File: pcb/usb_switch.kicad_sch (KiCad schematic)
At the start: 1 part, among them U2 FE1.1s

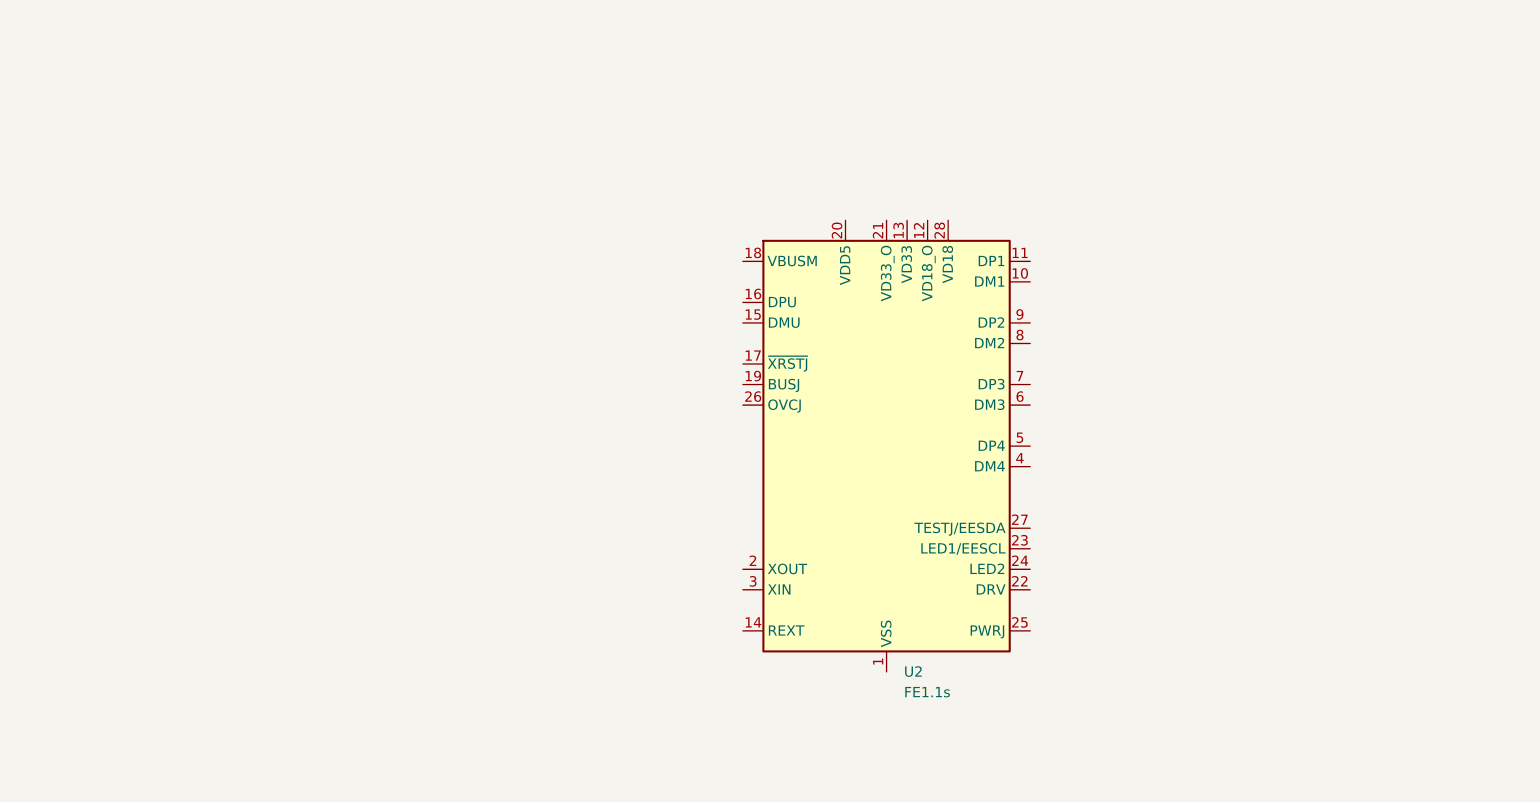
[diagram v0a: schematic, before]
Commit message: Schematic design
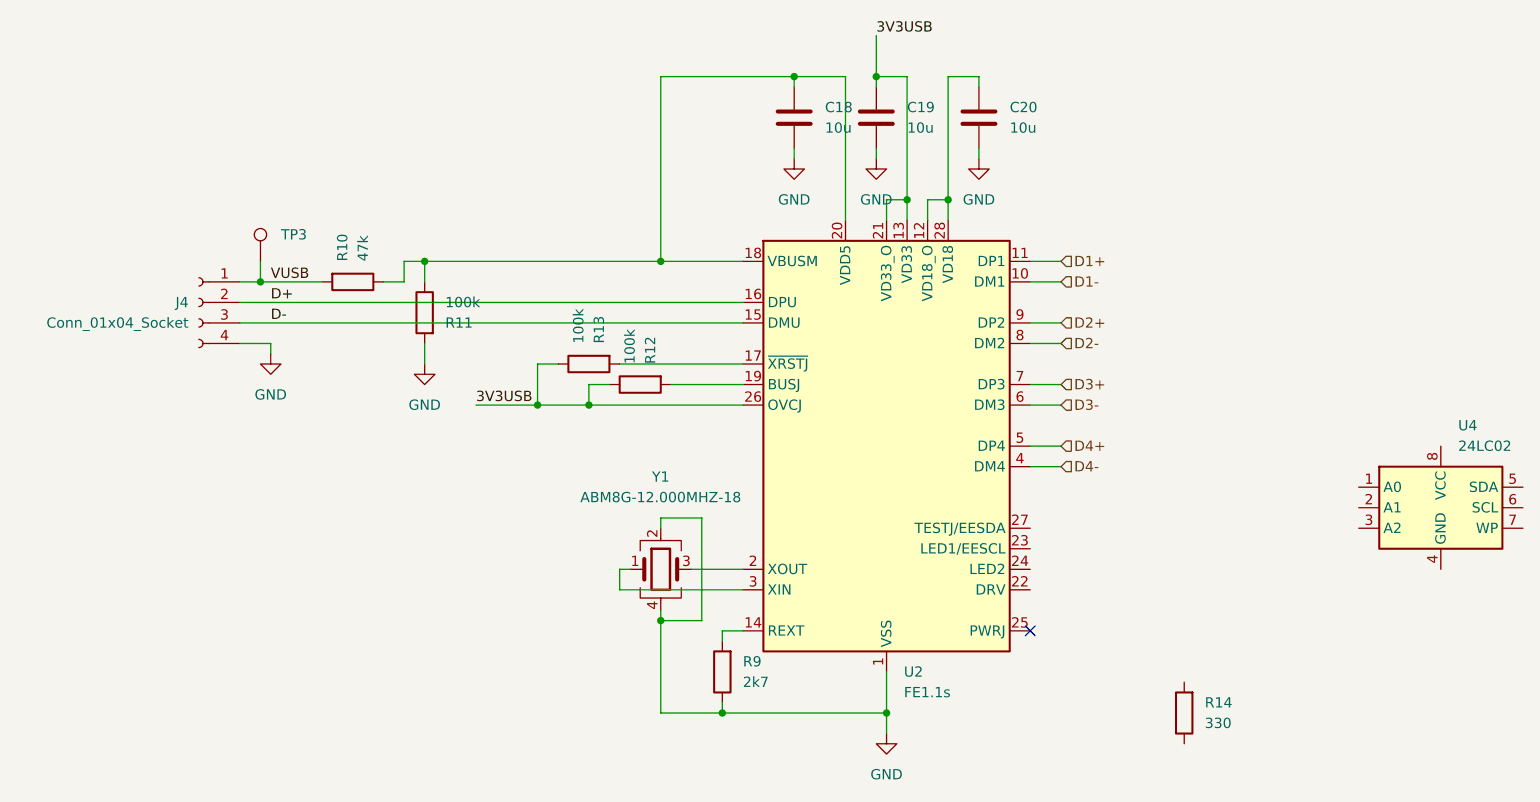
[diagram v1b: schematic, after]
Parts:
- added C18, C19, C20: 10u, Capacitor_SMD:C_1206_3216Metric_Pad1.33x1.80mm_HandSolder, symbol Device:C
- added J4: Conn_01x04_Socket, Connector_JST:JST_PH_B4B-PH-K_1x04_P2.00mm_Vertical, symbol Connector:Conn_01x04_Socket
- added R10: 47k, Resistor_SMD:R_0603_1608Metric_Pad0.98x0.95mm_HandSolder, symbol Device:R
- added R11, R12, R13: 100k, Resistor_SMD:R_0603_1608Metric_Pad0.98x0.95mm_HandSolder, symbol Device:R
- added R14: 330, Resistor_SMD:R_0603_1608Metric_Pad0.98x0.95mm_HandSolder, symbol Device:R
- added R9: 2k7, Resistor_SMD:R_0603_1608Metric_Pad0.98x0.95mm_HandSolder, symbol Device:R
- added TP3: TestPoint, TestPoint:TestPoint_Pad_D1.0mm, symbol Connector:TestPoint
- added U4: 24LC02, Package_SO:SOIC-8_3.9x4.9mm_P1.27mm, symbol Memory_EEPROM:24LC02
- added Y1: ABM8G-12.000MHZ-18, Crystal:Crystal_SMD_Abracon_ABM8G-4Pin_3.2x2.5mm, symbol Device:Crystal_GND24
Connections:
- net GND: now reaches U2.1 (VSS)
- net GND: now also C18.2, C19.2, C20.2, J4.4 (Pin_4), R11.2, R9.1, Y1.2, Y1.4
- net D1-: now reaches U2.10 (DM1)
- net D1+: now reaches U2.11 (DP1)
- net at U2.12 (VD18_O): now also U2.28 (VD18), C20.1
- net 3V3USB: now reaches U2.13 (VD33)
- net 3V3USB: now also U2.21 (VD33_O), U2.26 (OVCJ), C19.1, R12.1, R13.1
- net at U2.14 (REXT): now also R9.2
- net D-: now reaches U2.15 (DMU)
- net D-: now also J4.3 (Pin_3)
- net D+: now reaches U2.16 (DPU)
- net D+: now also J4.2 (Pin_2)
- net at U2.17 (~{XRSTJ}): now also R13.2
- net at U2.18 (VBUSM): now also U2.20 (VDD5), C18.1, R10.1, R11.1
- net at U2.19 (BUSJ): now also R12.2
- net at U2.2 (XOUT): now also Y1.3
- net at U2.3 (XIN): now also Y1.1
- net D4-: now reaches U2.4 (DM4)
- net D4+: now reaches U2.5 (DP4)
- net D3-: now reaches U2.6 (DM3)
- net D3+: now reaches U2.7 (DP3)
- net D2-: now reaches U2.8 (DM2)
- net D2+: now reaches U2.9 (DP2)
- new net VUSB: J4.1 (Pin_1), R10.2, TP3.1
- no-connect marks 0 -> 1
